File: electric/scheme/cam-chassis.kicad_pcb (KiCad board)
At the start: 2 copper layers, 51.5 x 34.6 mm, 45 parts, among them IC1 ATMEGA8-AI, K1 pyro, P1 TST, P2 TST, P3 TST, P4 TST, P5 TST, P6 TST, P7 servo, Q3 bc857, Q4 bc847, Q5 irlml2244, Q6 NPN, Q7 irlml2244, U1 MINI-USB-B-4-bases, Y1 Crystal

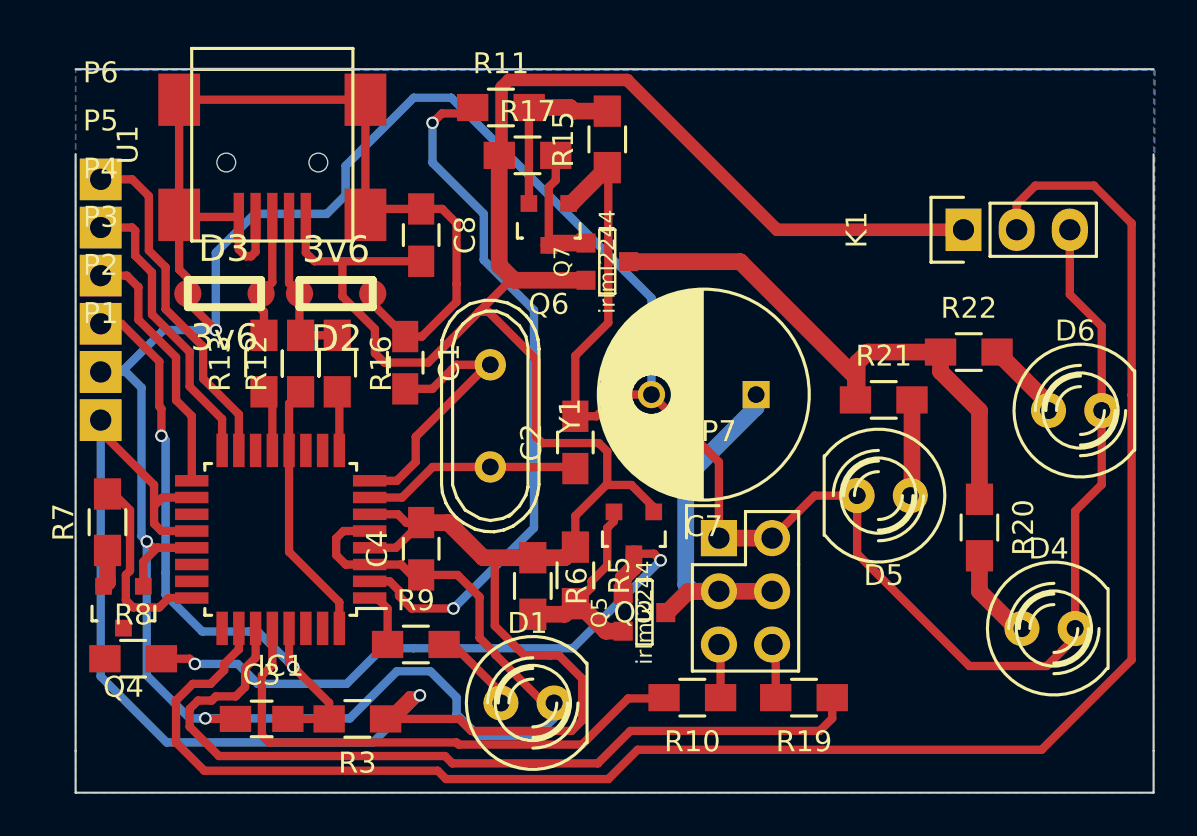
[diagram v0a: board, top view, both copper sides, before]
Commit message: Prepared SVG.
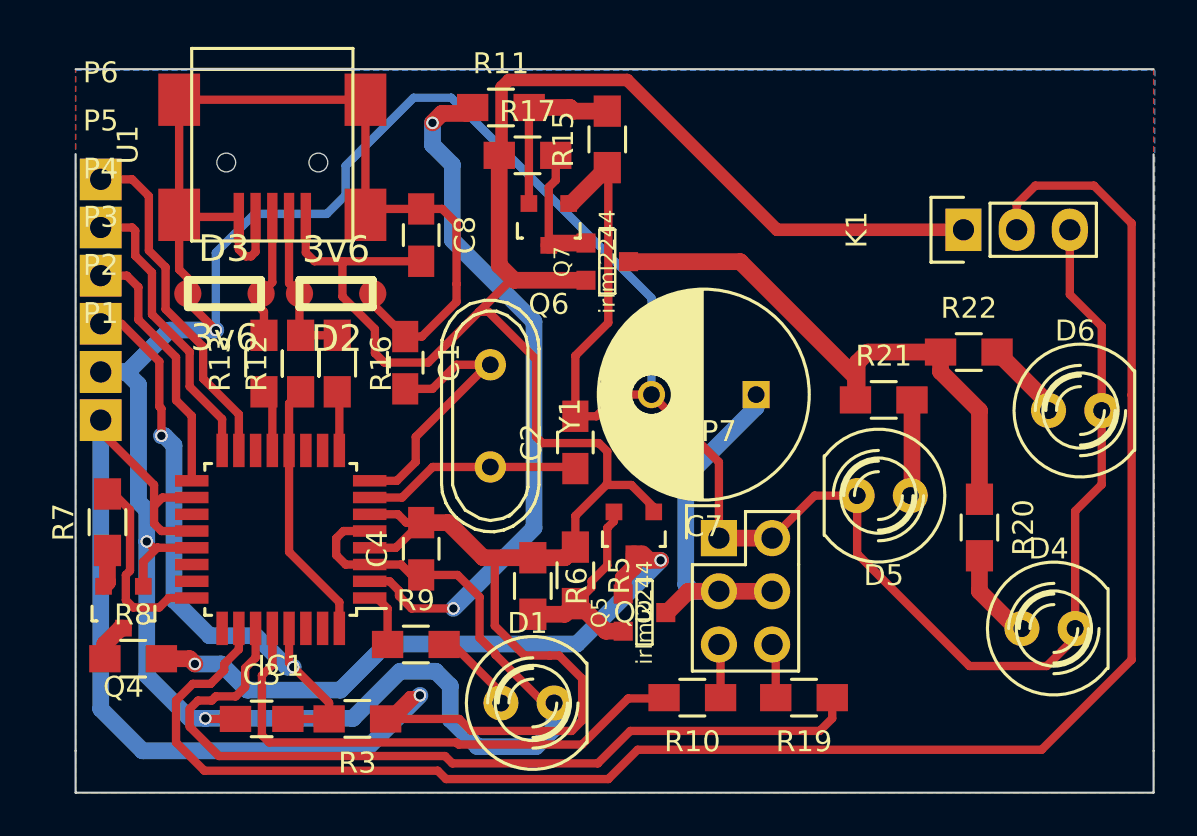
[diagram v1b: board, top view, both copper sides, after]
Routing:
- net GND: track 225.5 -> 244.2 mm
- net Net-(Q4-Pad3): track 0.00 -> 1.90 mm
- net /gate: track 30.3 -> 31.9 mm
- net VCC: track 158.8 -> 160.0 mm
